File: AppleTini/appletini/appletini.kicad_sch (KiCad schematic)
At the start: 4 parts, among them J1 Conn_02x25_Counter_Clockwise, Q1 DMG2305UX-7, U16 Pico, U17 Teensy4.1

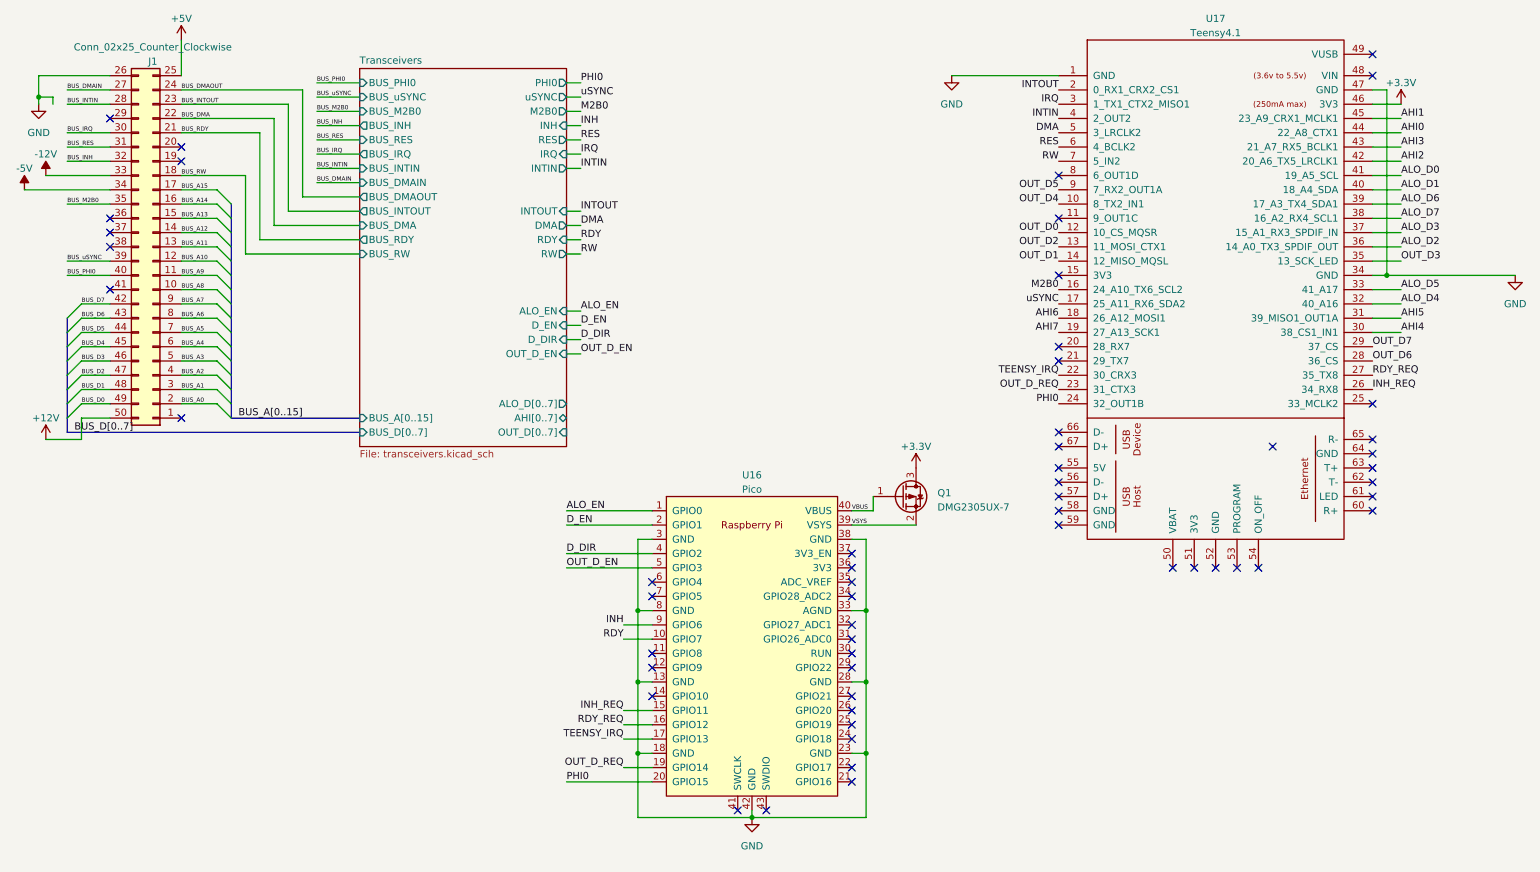
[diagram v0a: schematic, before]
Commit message: part picks and cleanup
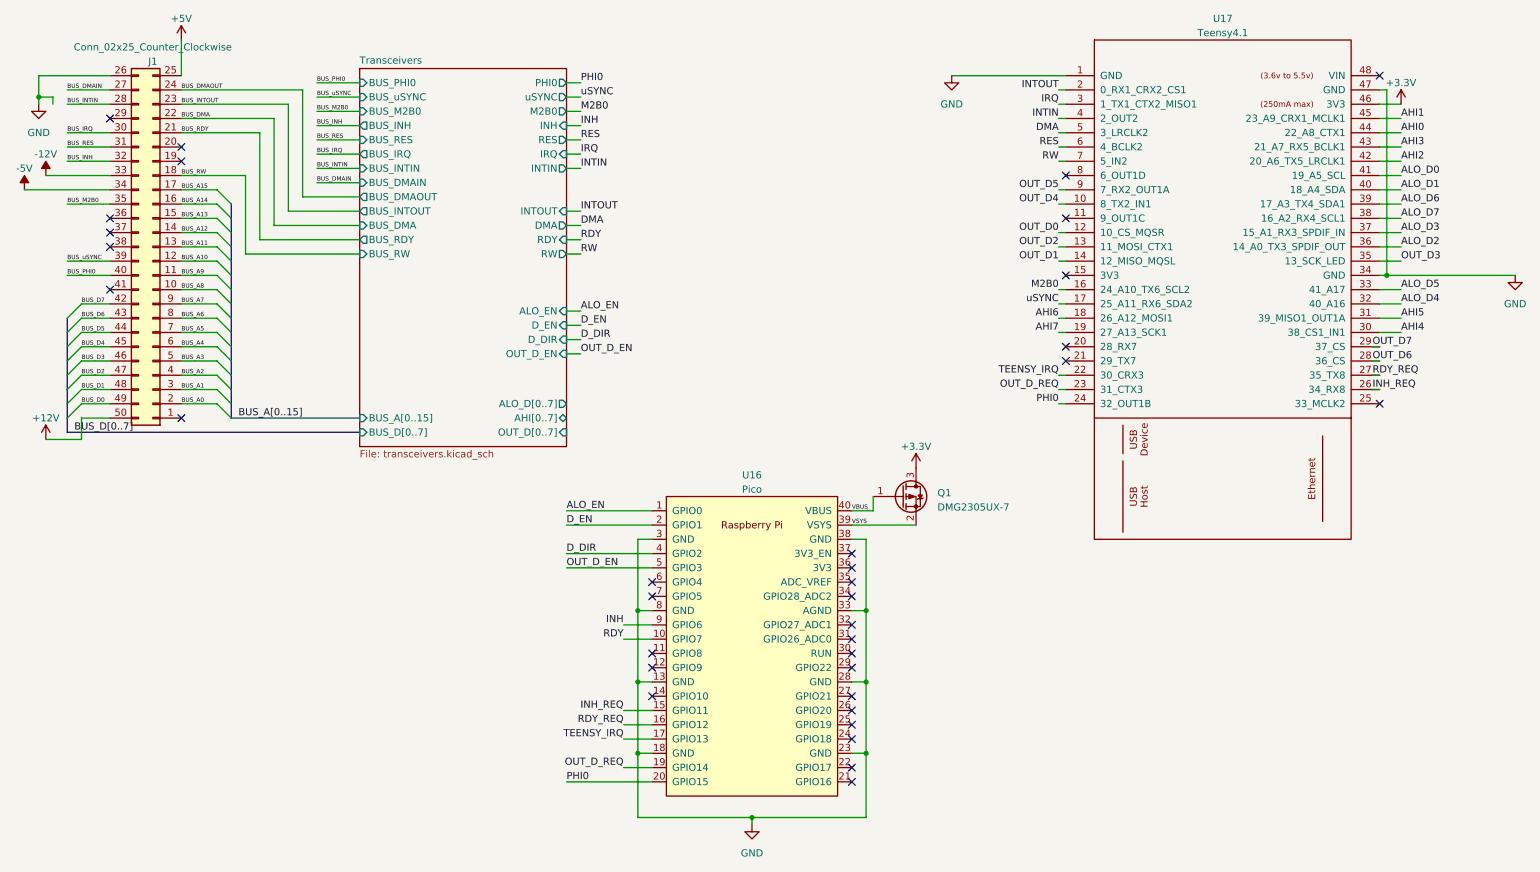
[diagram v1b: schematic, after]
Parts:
- Q1: LCSC (none) -> C5261054
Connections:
- net GND: no longer U16.42 (GND)
- no-connect marks 56 -> 34
